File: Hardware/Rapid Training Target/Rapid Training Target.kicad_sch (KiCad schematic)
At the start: 15 parts, among them Q1 2N7002, Q2 2N7002, Q3 2N7002

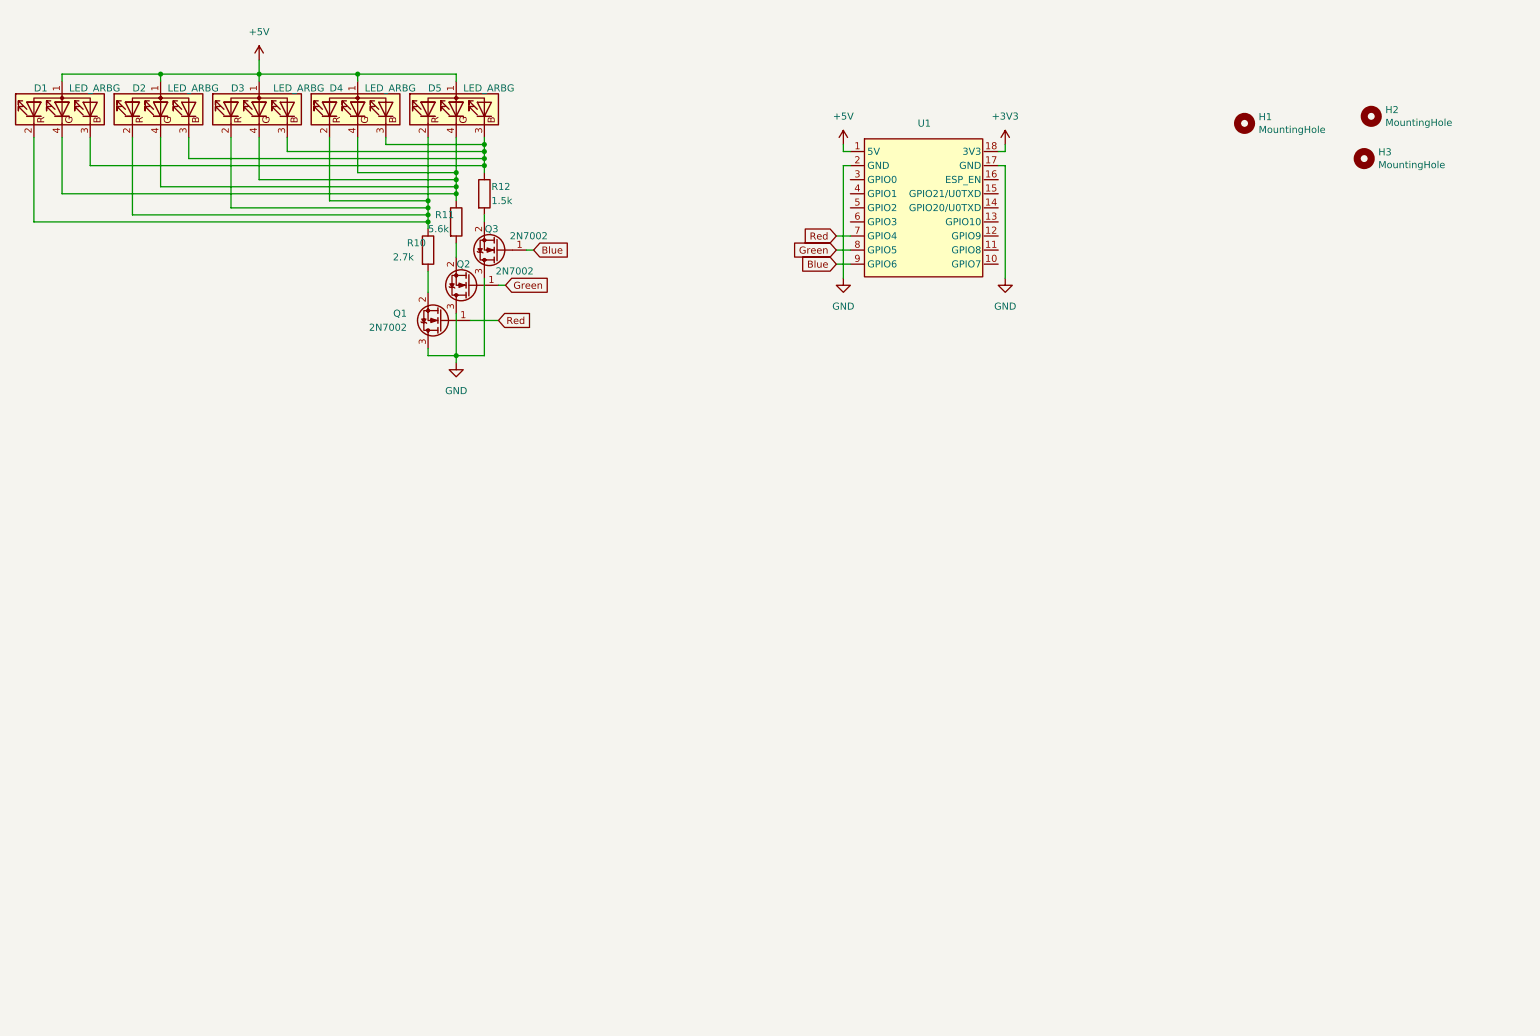
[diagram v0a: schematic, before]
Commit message: added code and remote
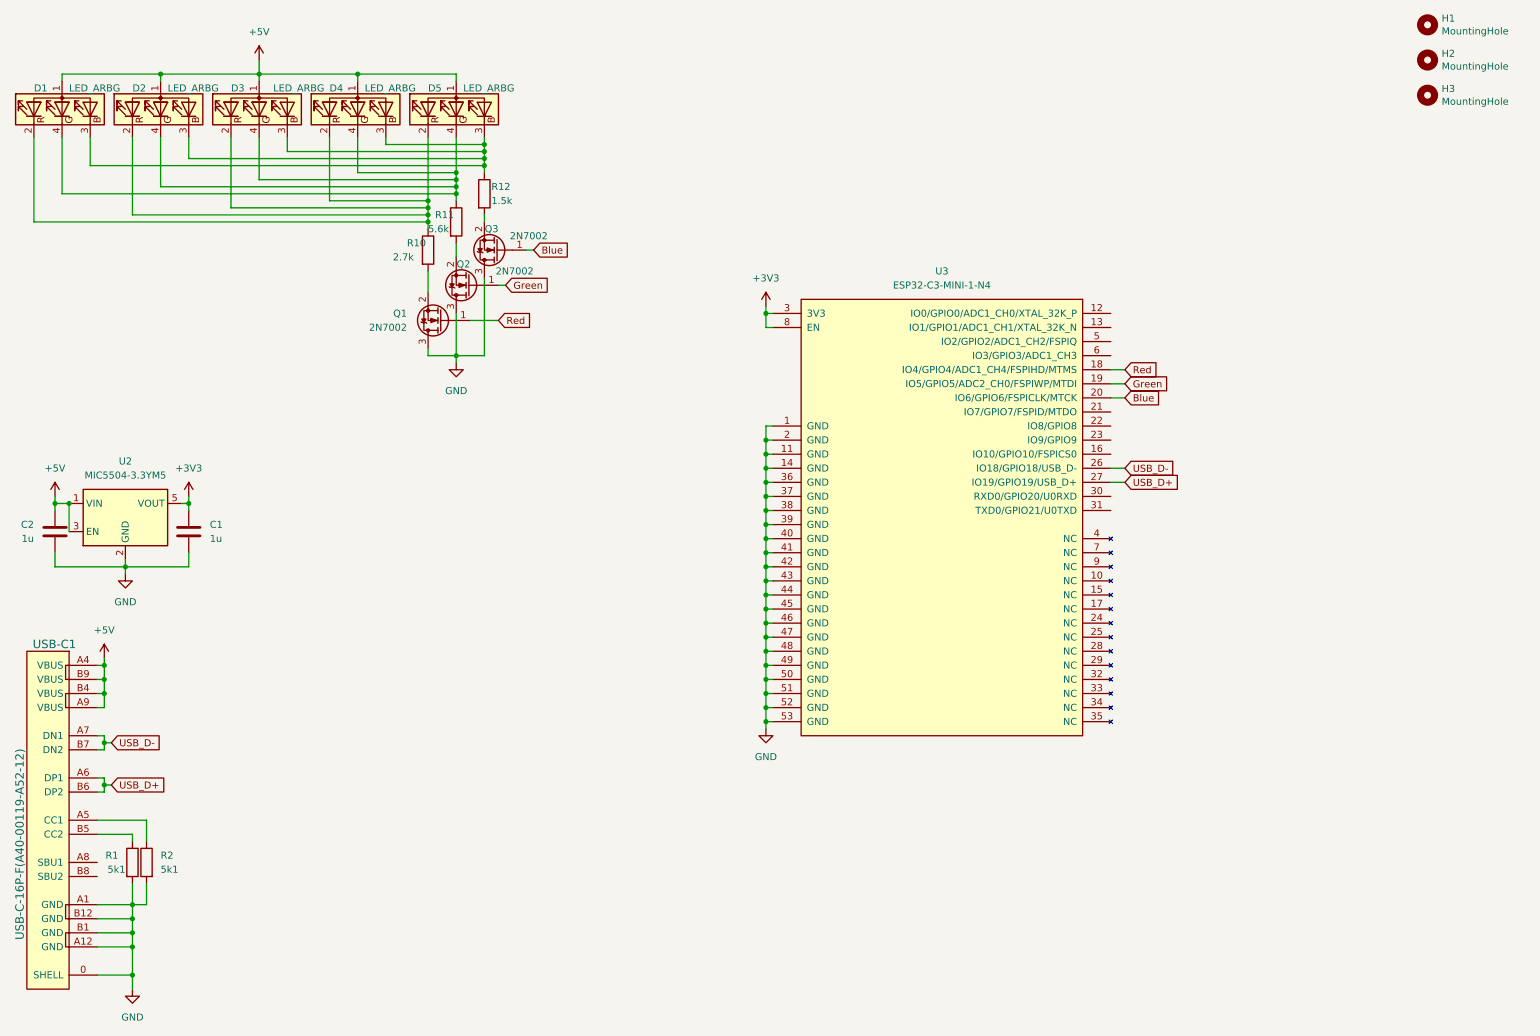
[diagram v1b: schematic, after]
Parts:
- removed U1: ~, Personal:ESP32-C3-DevKit, symbol personal2:ESP32-C3_DevKit_Rev_A
- added C1, C2: 1u, Capacitor_SMD:C_0603_1608Metric, symbol Device:C
- added R1, R2: 5k1, Resistor_SMD:R_0603_1608Metric, symbol Device:R
- added U2: MIC5504-3.3YM5, Package_TO_SOT_SMD:SOT-23-5, symbol Regulator_Linear:MIC5504-3.3YM5
- added U3: ESP32-C3-MINI-1-N4, Personal:ESP32-­C3-­MINI­-1, symbol personal2:ESP32-­C3-­MINI­-1
- added USB-C1: USB-C-16P-F(A40-00119-A52-12), Personal:USB2.0_TYPE-C(A40-00119-A52-12), symbol personal2:USB2.0_TYPE-C(A40-00119-A52-12)
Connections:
- net +3V3: now also C1.1, U2.5 (VOUT), U3.3 (3V3), U3.8 (EN)
- net +5V: now also C2.1, U2.1 (VIN), U2.3 (EN), USB-C1.A4 (VBUS), USB-C1.A9 (VBUS), USB-C1.B4 (VBUS), USB-C1.B9 (VBUS)
- net Blue: now also U3.20 (IO6/GPIO6/FSPICLK/MTCK)
- net GND: now also C1.2, C2.2, R1.2, R2.2, U2.2 (GND), U3.1 (GND), U3.11 (GND), U3.14 (GND), U3.2 (GND), U3.36 (GND), U3.37 (GND), U3.38 (GND), U3.39 (GND), U3.40 (GND), U3.41 (GND), U3.42 (GND), U3.43 (GND), U3.44 (GND), U3.45 (GND), U3.46 (GND), U3.47 (GND), U3.48 (GND), U3.49 (GND), U3.50 (GND), U3.51 (GND), U3.52 (GND), U3.53 (GND), USB-C1.0 (SHELL), USB-C1.A1 (GND), USB-C1.A12 (GND), USB-C1.B1 (GND), USB-C1.B12 (GND)
- net Green: now also U3.19 (IO5/GPIO5/ADC2_CH0/FSPIWP/MTDI)
- net Red: now also U3.18 (IO4/GPIO4/ADC1_CH4/FSPIHD/MTMS)
- new net: R2.1, USB-C1.A5 (CC1)
- new net: R1.1, USB-C1.B5 (CC2)
- new net USB_D+: U3.27 (IO19/GPIO19/USB_D+), USB-C1.A6 (DP1), USB-C1.B6 (DP2)
- new net USB_D-: U3.26 (IO18/GPIO18/USB_D-), USB-C1.A7 (DN1), USB-C1.B7 (DN2)
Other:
- moved on the sheet: H1, H2, H3
